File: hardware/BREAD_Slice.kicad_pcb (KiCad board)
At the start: 2 copper layers, 70 x 100 mm, 16 parts, among them J1 Conn_01x10_Female, U1 AP63205

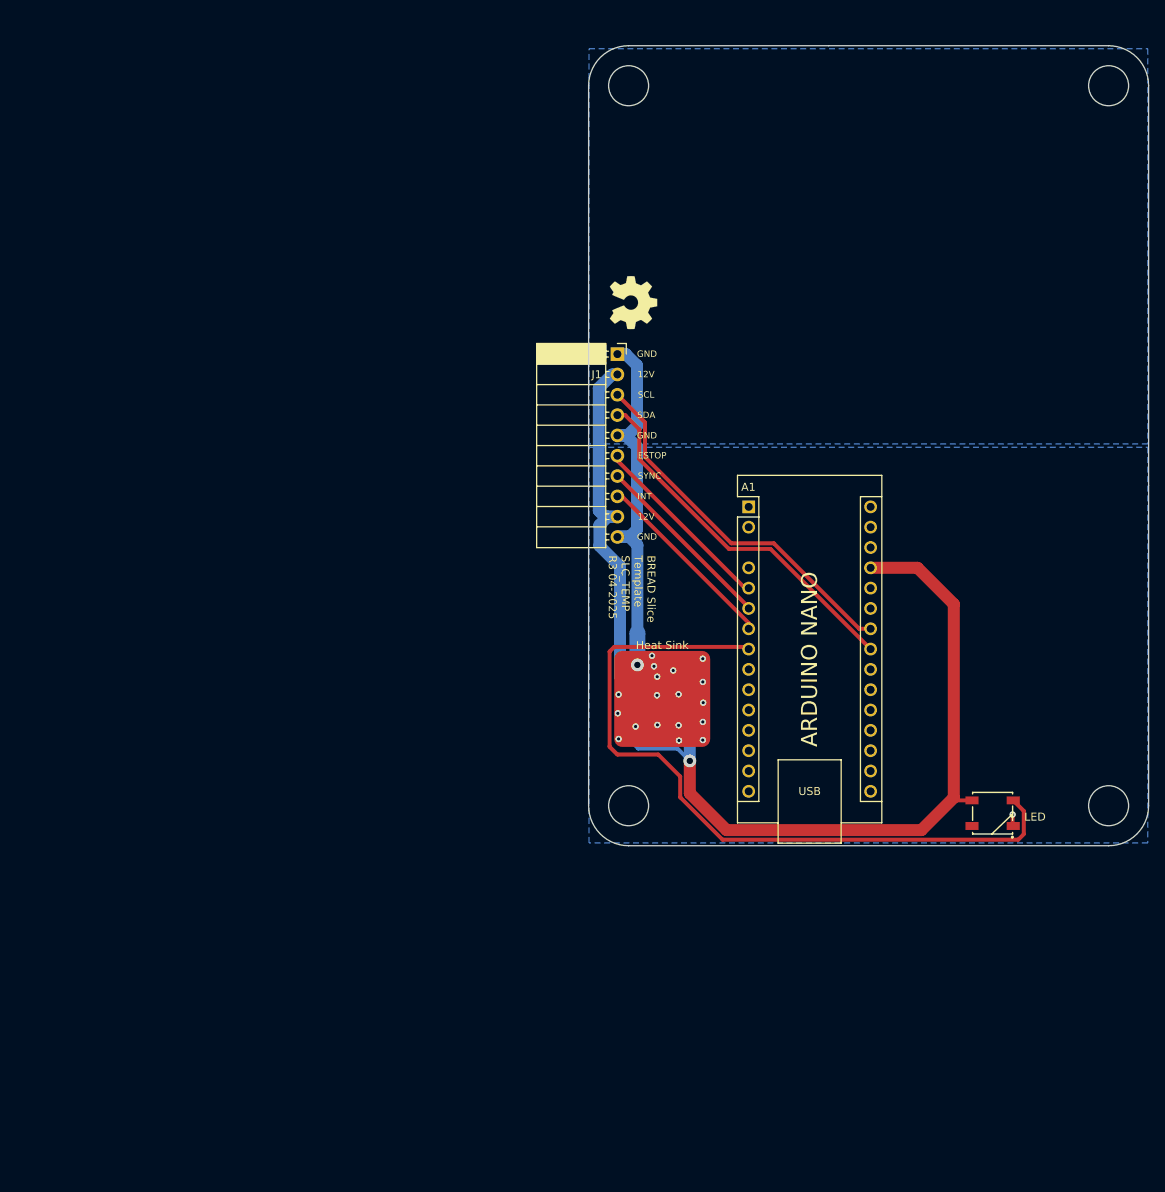
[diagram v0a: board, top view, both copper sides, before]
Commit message: initial commit post-fork from s2l
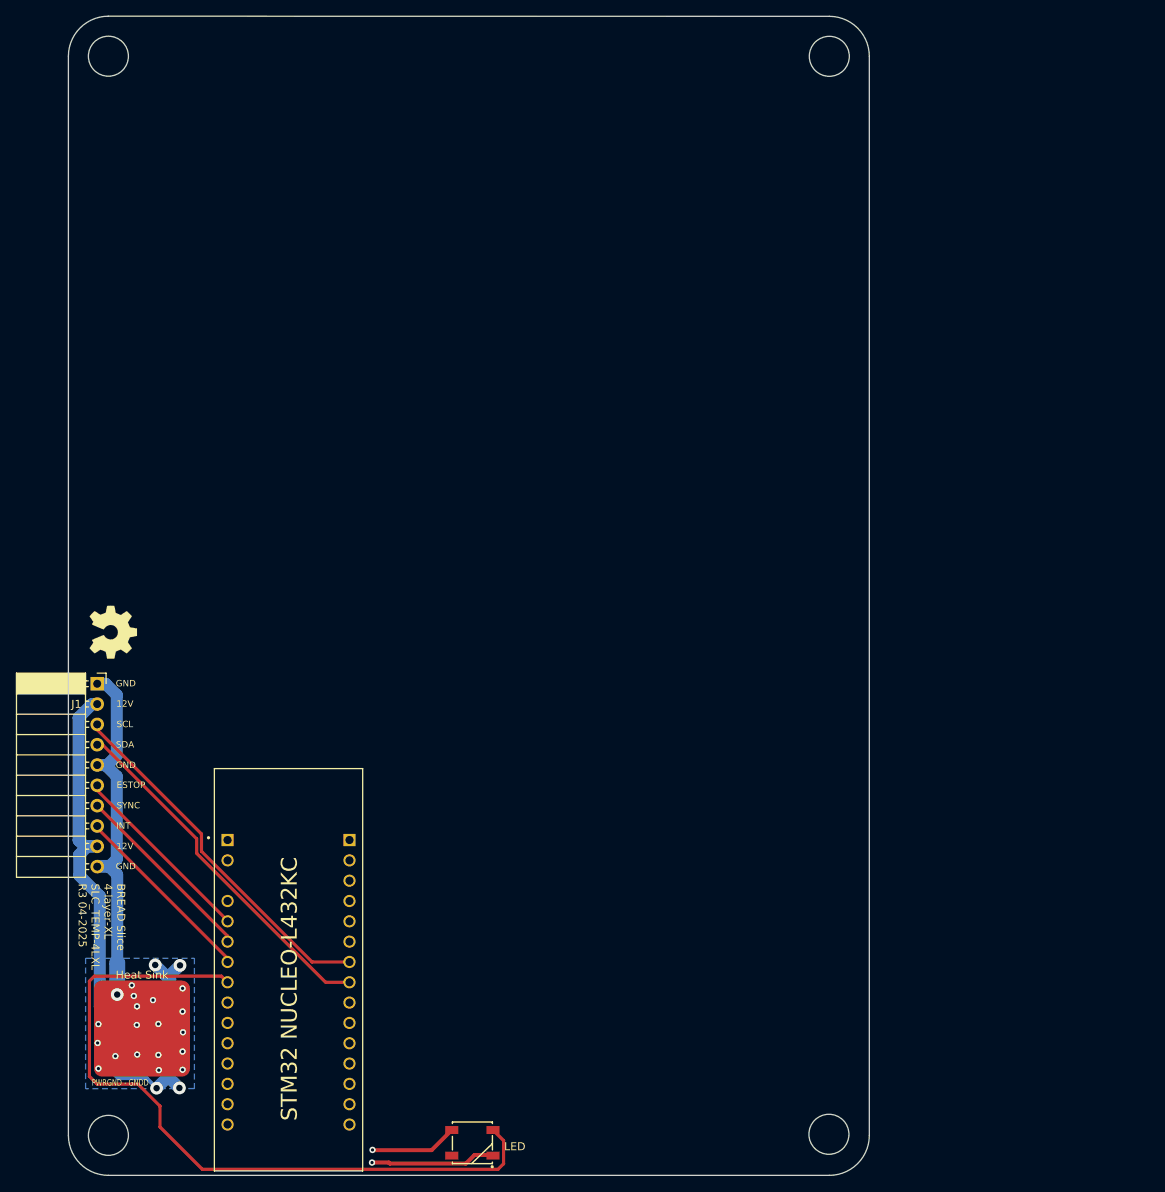
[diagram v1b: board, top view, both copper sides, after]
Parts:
- removed A1: Arduino_Nano_v3.x, Module:Arduino_Nano
- added U2: NUCLEO-L432KC, kml-custom:MODULE_NUCLEO-L432KC, F.Cu at (85.1, 155.3)
- moved C1 77.0 mm to (63.8, 160.7)
- moved C2 77.0 mm to (66.1, 167.5)
- moved D1 77.0 mm to (108.1, 176.9)
- moved J1 77.0 mm to (61.2, 119.6)
- moved L1 77.0 mm to (68.8, 164.0)
- moved U1 77.0 mm to (63.7, 164.0)
- moved C3 77.0 mm to (68.8, 160.7)
- moved HS1 77.0 mm to (66.8, 162.7)
- moved Logo1 77.0 mm to (63.2, 113.1)
- moved NT1 77.0 mm to (63.7, 156.4)
- moved C4 77.0 mm to (68.8, 157.6)
- moved H2 77.0 mm to (62.6, 176.0)
- moved H1 65.1 mm to (62.6, 41.1)
- moved H4 53.9 mm to (152.6, 175.9)
- moved H3 35.1 mm to (152.7, 41.1)
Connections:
- net +5V renamed +5VD
- net GND renamed GNDD
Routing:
- net +5VD: track 104.2 -> 42.1 mm, vias 1 -> 5
- net GNDD: track 16.8 -> 31.0 mm
- net /I2C_DAT: track 46.0 -> 44.9 mm
- net /I2C_CLK: track 46.3 -> 45.5 mm
- added copper zone on In2.Cu, net +12V
- added copper zone on In2.Cu, net +5VD
- added copper zone on In1.Cu, net GNDD
- added copper zone on In1.Cu, net GNDPWR
- removed copper zone on B.Cu, net GNDPWR
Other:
- board size 70 x 100 mm -> 100.1 x 144.9 mm
- copper layers 2 -> 4
- board text added: "12V->5V Sw.Reg"
- board text added: "BREAD Slice 4-layer-XL SLC_TEMP-4LXL R3 04-2025"
- board text added: "L1 (Top): - Template digital components (Nano, RGB LED) and I²C signals - use minimal ground pours. L2 (Inner 1): - Solid ground plane - split into an upper {dblquote}gndpwr{dblquote} zone (handling 12V returns) and a lower digital ground zone, connected only at the regulator - these can be resized to accommadate additional planes - i.e. decreasing 12V/GNDPWR planes to connector edge and creating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"
- board text added: "PWRGND - GNDD"
- board text added: "STM32 NUCLEO-L432KC"
- board text removed: "12V->5V Reg"
- board text removed: "ARDUINO NANO"
- board text removed: "BREAD Slice Template SLC_TEMP R3 04-2025"
